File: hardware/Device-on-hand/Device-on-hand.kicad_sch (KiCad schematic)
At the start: 4 parts, among them J1 Screw_Terminal_01x02, U1 module_mpu6050, U2 mini_esp32

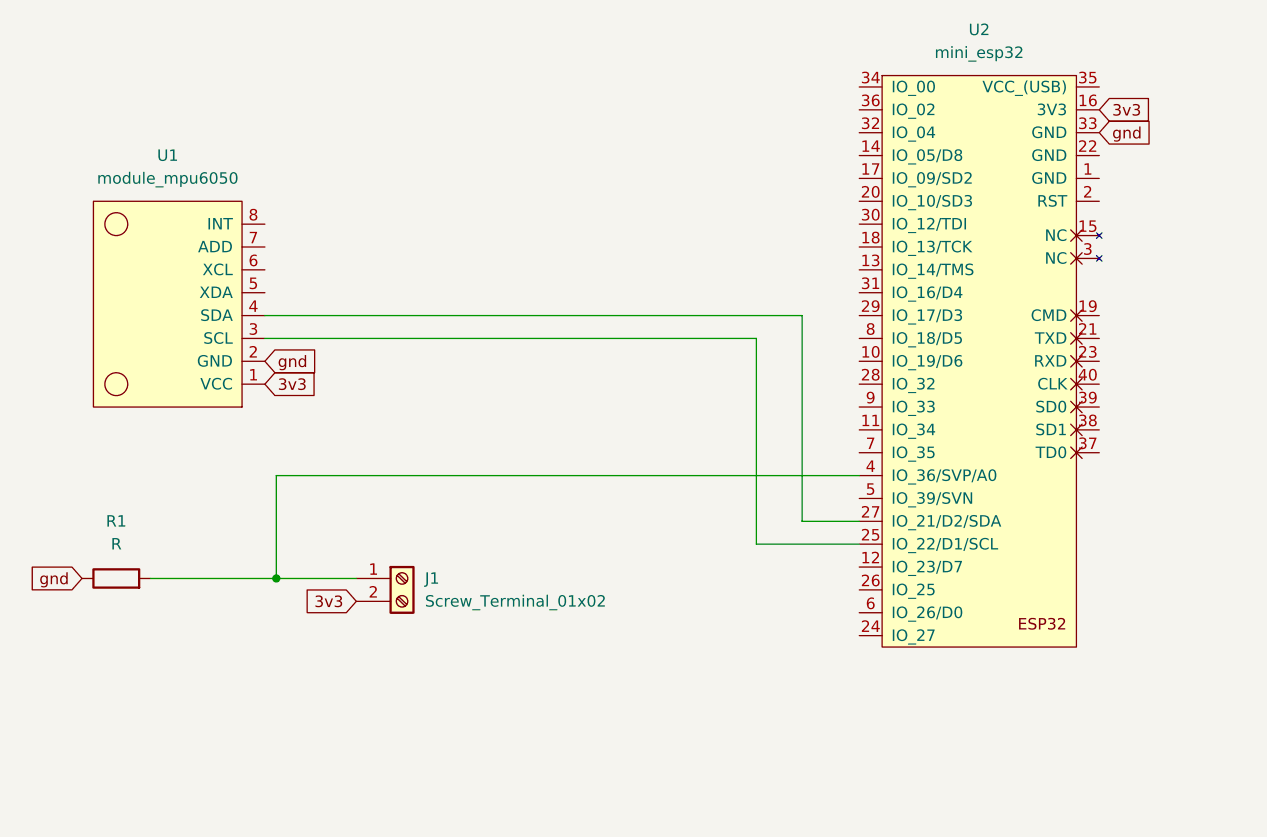
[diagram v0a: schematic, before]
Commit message: update
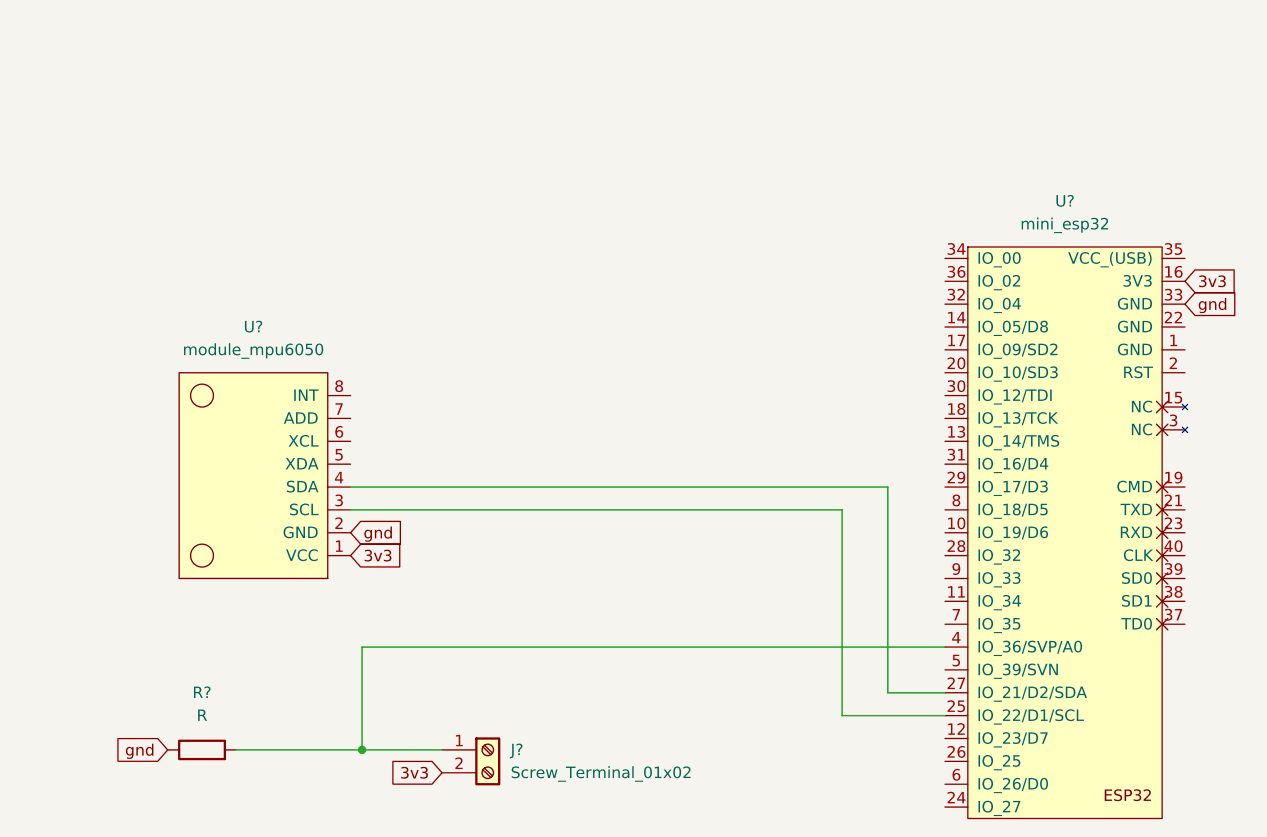
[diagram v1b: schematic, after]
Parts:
- removed J1: Screw_Terminal_01x02, Connector_Phoenix_MSTB:PhoenixContact_MSTBA_2,5_2-G-5,08_1x02_P5.08mm_Horizontal, symbol Connector:Screw_Terminal_01x02
- removed R1: R, Resistor_THT:R_Axial_DIN0207_L6.3mm_D2.5mm_P10.16mm_Horizontal, symbol Device:R
- removed U1: module_mpu6050, usini_sensors:module_mpu6050, symbol usini_sensors:module_mpu6050
- removed U2: mini_esp32, ESP32_mini:ESP32_mini, symbol ESP32_mini:mini_esp32
- added J?: Screw_Terminal_01x02, Connector_Phoenix_MSTB:PhoenixContact_MSTBA_2,5_2-G-5,08_1x02_P5.08mm_Horizontal, symbol Connector:Screw_Terminal_01x02
- added R?: R, Resistor_THT:R_Axial_DIN0207_L6.3mm_D2.5mm_P10.16mm_Horizontal, symbol Device:R
- added U?: module_mpu6050, usini_sensors:module_mpu6050, symbol usini_sensors:module_mpu6050
- added U?: mini_esp32, ESP32_mini:ESP32_mini, symbol ESP32_mini:mini_esp32
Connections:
- net 3v3: now also J?.2 (Pin_2), U?.1 (VCC), U?.16 (3V3)
- net gnd: now also R?.1, U?.2 (GND), U?.33 (GND)
- new net: U?.25 (IO_22/D1/SCL), U?.3 (SCL)
- new net: U?.27 (IO_21/D2/SDA), U?.4 (SDA)
- new net: J?.1 (Pin_1), R?.2, U?.4 (IO_36/SVP/A0)
